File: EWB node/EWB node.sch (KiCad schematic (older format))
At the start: 35 parts, among them J1 USB_A, J2 Barrel_Jack_Switch, J3 AVR-ISP-6, J4 Conn_01x06, P1 USB_C_Plug_USB2.0, SW1 SW_SPST, SW2 SW_Push_Dual, U1 RFM95W-915S2, U2 USBLC6-2P6, U3 ATmega328P-AU, U4 NCP1117-5.0_TO252, U5 LP2985-3.3, Y1 16MHz

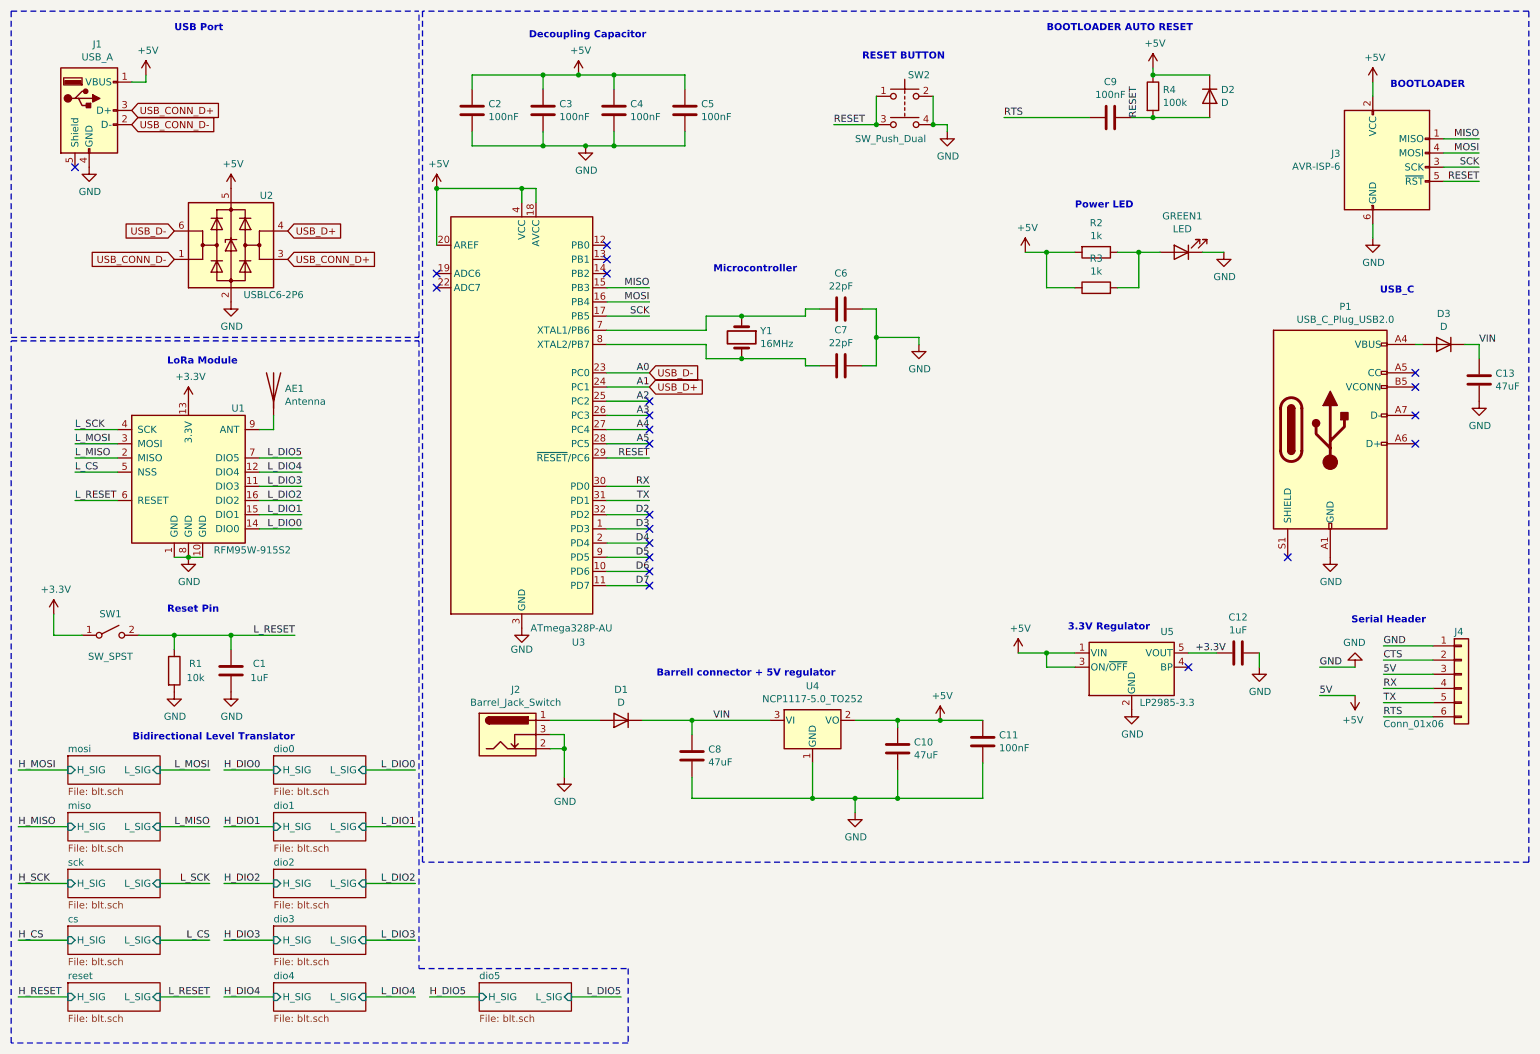
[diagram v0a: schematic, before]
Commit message: pcb layout
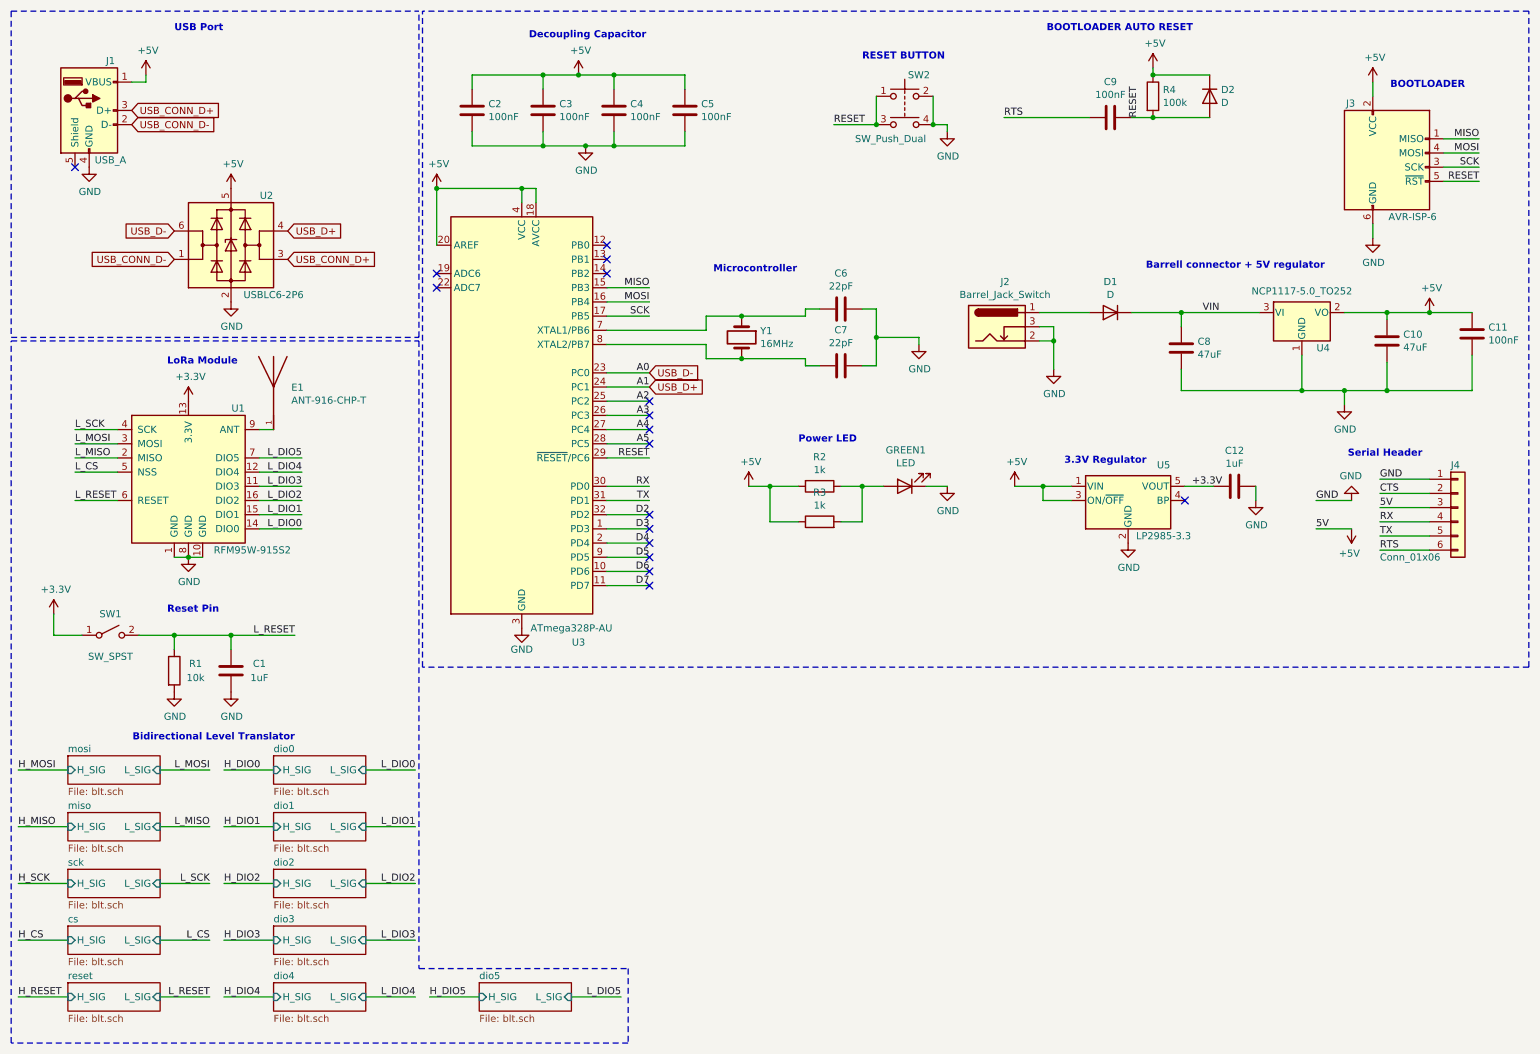
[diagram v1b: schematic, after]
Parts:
- removed AE1: Antenna, symbol Device:Antenna
- removed C13: 47uF, Capacitor_SMD:C_0201_0603Metric_Pad0.64x0.40mm_HandSolder, symbol Device:C
- removed D3: D, Diode_SMD:D_0201_0603Metric_Pad0.64x0.40mm_HandSolder, symbol Device:D
- removed P1: USB_C_Plug_USB2.0, symbol Connector:USB_C_Plug_USB2.0
- added E1: ANT-916-CHP-T, ant-916-chp-t:ant-916-chp-t, symbol ANT-916-CHP-T:ANT-916-CHP-T
- C1, C10, C11, C12, C2, C3, C4, C5, C6, C7, C8, C9: footprint Capacitor_SMD:C_0201_0603Metric_Pad0.64x0.40mm_HandSolder -> Capacitor_SMD:C_0603_1608Metric_Pad1.08x0.95mm_HandSolder
- J1: footprint (none) -> digikey-footprints:USB_A_Female_UE27AC54100
- J2: footprint (none) -> Connector_BarrelJack:BarrelJack_CUI_PJ-036AH-SMT_Horizontal
- J3, J4: footprint (none) -> Connector_PinHeader_2.54mm:PinHeader_1x06_P2.54mm_Vertical
- SW1: footprint (none) -> Button_Switch_SMD:SW_SPST_B3S-1000
- SW2: footprint (none) -> Button_Switch_SMD:SW_DIP_SPSTx02_Slide_6.7x6.64mm_W8.61mm_P2.54mm_LowProfile
- U1: footprint (none) -> RF_Module:HOPERF_RFM9XW_SMD
- Y1: footprint (none) -> Crystal:Crystal_SMD_0603-2Pin_6.0x3.5mm_HandSoldering
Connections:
- net at U1.9 (ANT): now also E1.1
- no-connect marks 22 -> 17
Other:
- note removed: "USB_C"
- moved on the sheet: C10, C11, C12, C8, D1, GREEN1, J2, J4, R2, R3, U4, U5
